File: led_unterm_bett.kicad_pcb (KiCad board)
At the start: 2 copper layers, 27 parts, among them J1 Conn_01x03, J2 Conn_01x03, J3 Conn_01x03, J4 Conn_01x02, J5 Screw_Terminal_01x02, J6 Conn_01x04, Q1 BSS138, Q2 BSS138, Q3 BSS138, U1 NodeMCU1.0(ESP-12E), U2 LM7805_TO220

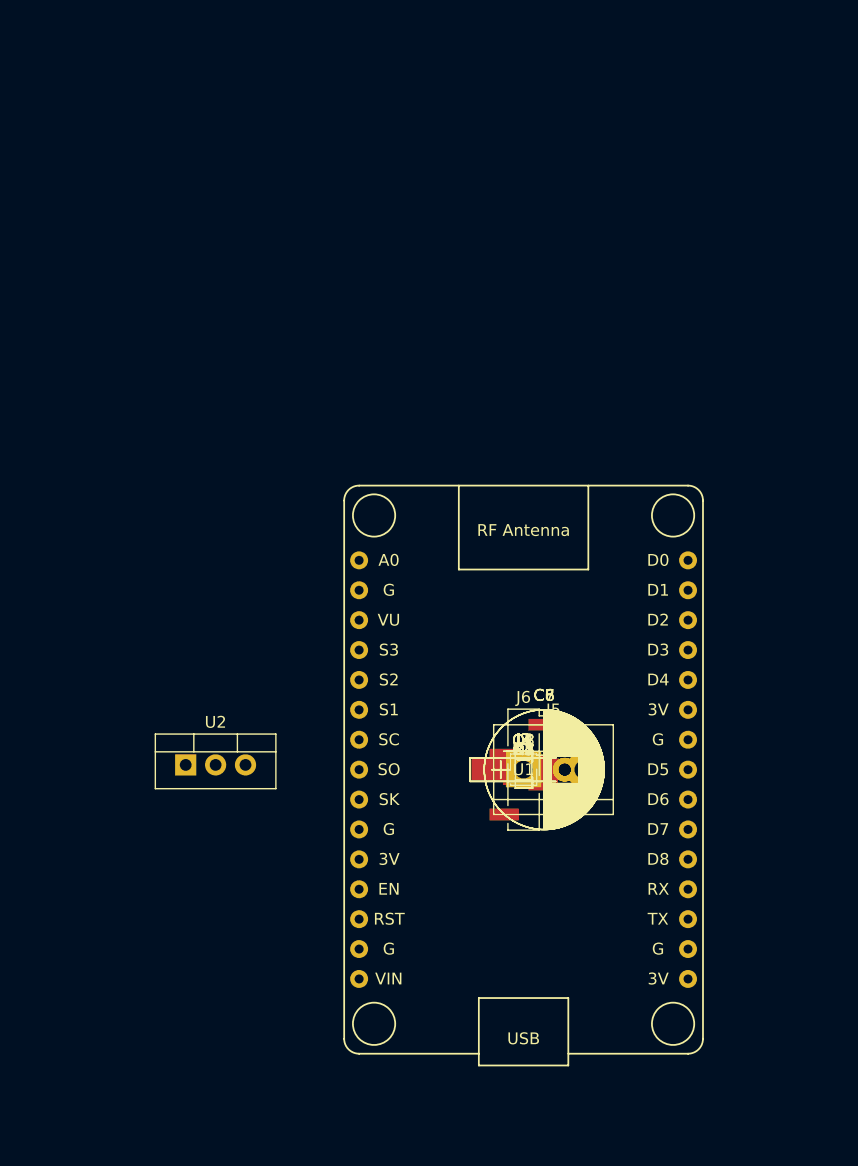
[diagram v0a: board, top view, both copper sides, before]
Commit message: placement complete
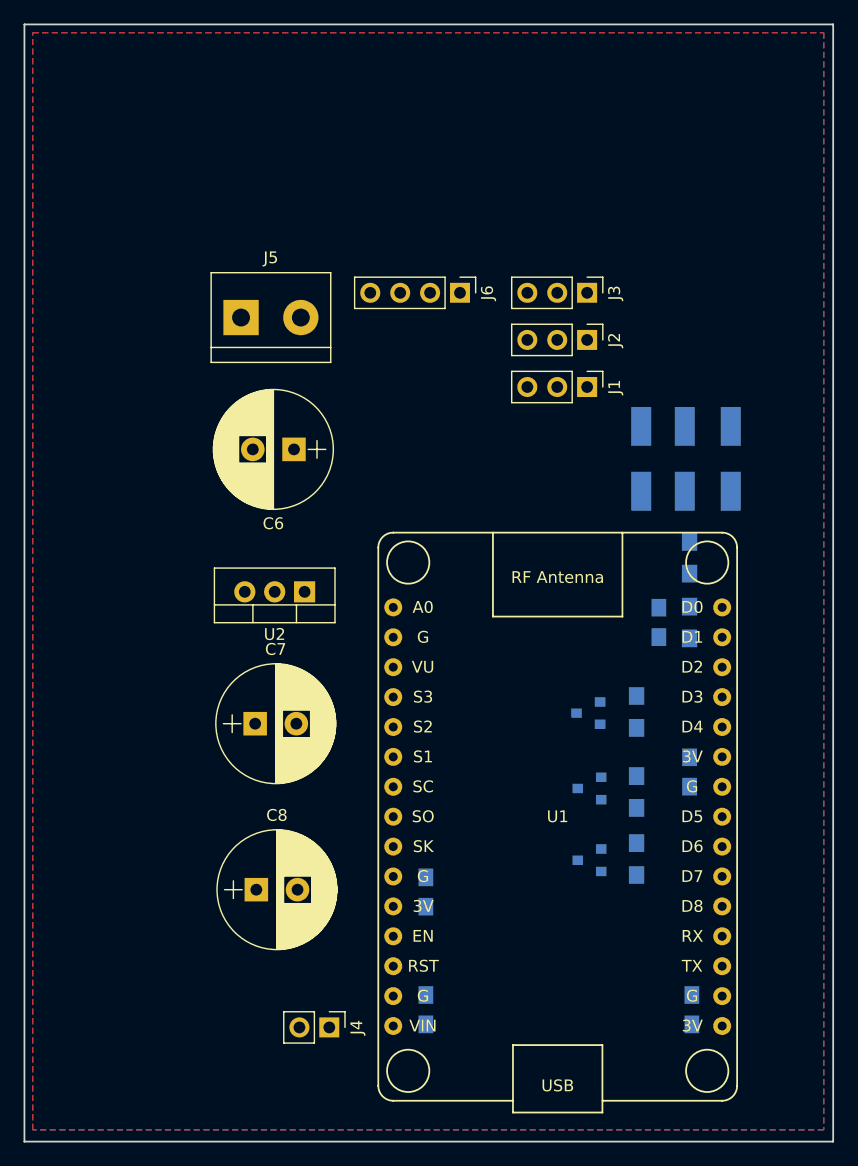
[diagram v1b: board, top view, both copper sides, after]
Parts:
- C1, C2, C3, C4, C5, D1, D2, D3, Q1, Q2, Q3, R1, R2, R3, R4, R5: moved to B.Cu
- J1, J3: footprint Pin_Headers:Pin_Header_Straight_1x03_Pitch1.00mm_SMD_Pin1Left -> Pin_Headers:Pin_Header_Straight_1x03_Pitch2.54mm
- J2: footprint Pin_Headers:Pin_Header_Straight_1x03_Pitch1.00mm_SMD_Pin1Right -> Pin_Headers:Pin_Header_Straight_1x03_Pitch2.54mm
- J4: footprint Pin_Headers:Pin_Header_Straight_1x02_Pitch1.27mm_SMD_Pin1Right -> Pin_Headers:Pin_Header_Straight_1x02_Pitch2.54mm
- J6: footprint Pin_Headers:Pin_Header_Straight_1x04_Pitch2.54mm_SMD_Pin1Right -> Pin_Headers:Pin_Header_Straight_1x04_Pitch2.54mm
- moved J5 45.3 mm to (124.5, 66.6)
- moved J6 40.9 mm to (143.1, 64.5), turned to 270 degrees
- moved J3 40.9 mm to (153.9, 64.5), turned to 270 degrees
- moved J2 36.9 mm to (153.9, 68.5), turned to 270 degrees
- moved C6 33.5 mm to (129.0, 77.8), turned to 180 degrees
- moved J1 32.9 mm to (153.9, 72.5), turned to 270 degrees
- moved D3 31.7 mm to (166.1, 78.6), turned to 90 degrees
- moved D2 29.7 mm to (162.2, 78.6), turned to 90 degrees
- moved D1 28.2 mm to (158.5, 78.6), turned to 90 degrees
- moved J4 27.4 mm to (132.0, 126.9), turned to 270 degrees
- moved C5 24.9 mm to (162.8, 125.4), turned to 270 degrees
- moved C8 24.9 mm to (125.8, 115.2)
- moved C7 23.1 mm to (125.7, 101.1)
- moved R1 22.9 mm to (162.6, 87.0), turned to 270 degrees
- moved C3 22.0 mm to (140.2, 125.4), turned to 90 degrees
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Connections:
- J1 pad 1: GND -> Net-(D1-Pad2)
- J1 pad 2: Net-(D1-Pad2) -> +5V
- J1 pad 3: +5V -> GND
- J2 pad 1: GND -> Net-(D2-Pad2)
- J2 pad 2: Net-(D2-Pad2) -> +5V
- J2 pad 3: +5V -> GND
- J3 pad 1: GND -> Net-(D3-Pad2)
- J3 pad 2: Net-(D3-Pad2) -> +5V
- J3 pad 3: +5V -> GND
- J6 pad 1: +12V -> Net-(J6-Pad1)
- J6 pad 4: Net-(J6-Pad4) -> +12V
- Q1 pad 3: Net-(J6-Pad2) -> Net-(J6-Pad1)
- Q2 pad 3: Net-(J6-Pad3) -> Net-(J6-Pad2)
- Q3 pad 3: Net-(J6-Pad4) -> Net-(J6-Pad3)
- U1 pad 1: Net-(U1-Pad1) -> (no net)
- U1 pad 13: Net-(U1-Pad13) -> (no net)
- U1 pad 18: Net-(U1-Pad18) -> (no net)
- U1 pad 19: Net-(U1-Pad19) -> (no net)
- U1 pad 2: Net-(U1-Pad2) -> (no net)
- U1 pad 20: Net-(U1-Pad20) -> (no net)
- U1 pad 21: Net-(U1-Pad21) -> (no net)
- U1 pad 27: Net-(U1-Pad27) -> (no net)
- U1 pad 28: Net-(U1-Pad28) -> (no net)
- U1 pad 29: Net-(U1-Pad29) -> (no net)
- U1 pad 3: Net-(U1-Pad3) -> (no net)
- U1 pad 4: Net-(U1-Pad4) -> (no net)
- U1 pad 5: Net-(U1-Pad5) -> (no net)
- U1 pad 6: Net-(U1-Pad6) -> (no net)
- U1 pad 7: Net-(U1-Pad7) -> (no net)
- U1 pad 8: Net-(U1-Pad8) -> (no net)
- U1 pad 9: Net-(U1-Pad9) -> (no net)
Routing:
- added copper zone on B.Cu, net GND
- added copper zone on F.Cu, net GND
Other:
- board outline added: 68.7 x 94.9 mm
